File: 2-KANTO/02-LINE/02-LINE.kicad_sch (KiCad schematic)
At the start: 74 parts, among them J2 WRITER CONN, J3 Conn_01x05, U1 STM32F446RETx

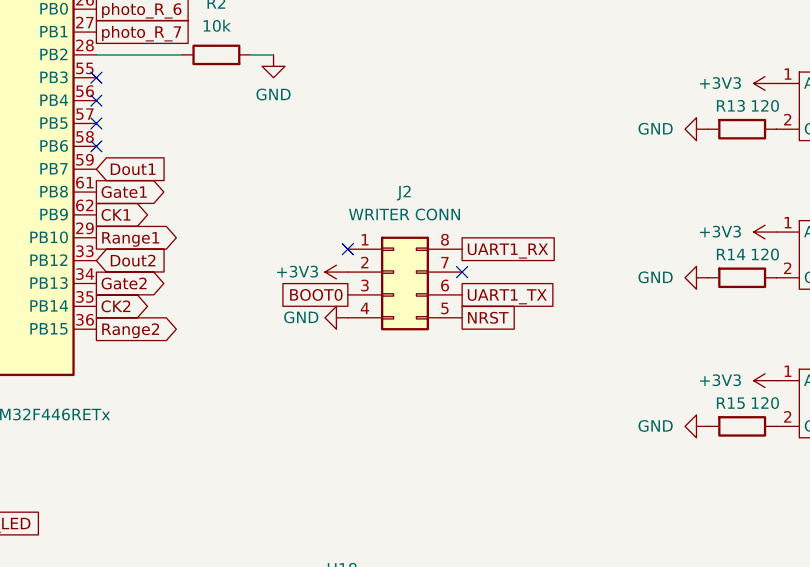
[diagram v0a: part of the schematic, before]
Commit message: mike
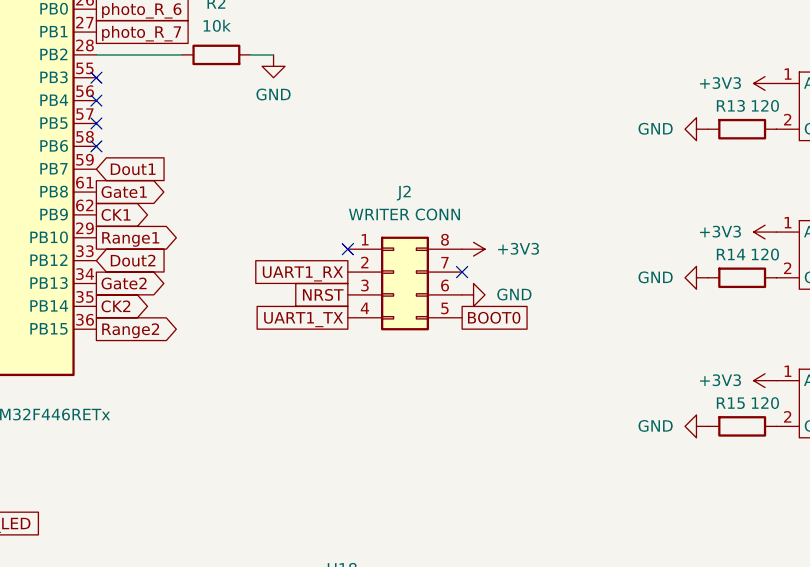
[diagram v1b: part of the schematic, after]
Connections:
- net +3V3: now also J2.8 (Pin_8); no longer J2.2 (Pin_2)
- net BOOT0: now also J2.5 (Pin_5); no longer J2.3 (Pin_3)
- net GND: now also J2.6 (Pin_6); no longer J2.4 (Pin_4)
- net NRST: now also J2.3 (Pin_3); no longer J2.5 (Pin_5)
- net UART1_RX: now also J2.2 (Pin_2); no longer J2.8 (Pin_8)
- net UART1_TX: now also J2.4 (Pin_4); no longer J2.6 (Pin_6)
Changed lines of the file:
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@@
     )
   )
-  (global_label "BOOT0" (shape passive) (at 113.665 124.46 180) (fields_autoplaced)
+  (global_label "UART1_TX" (shape passive) (at 113.665 127 180) (fields_autoplaced)
     (effects (font (size 1.27 1.27)) (justify right))
-    (property "Intersheetrefs" "${INTERSHEET_REFS}" (at 105.683 124.46 0)
+    (property "Intersheetrefs" "${INTERSHEET_REFS}" (at 102.7802 127 0)
       (effects (font (size 1.27 1.27)) (justify right) hide)
     )
@@
     )
   )
-  (global_label "UART1_TX" (shape passive) (at 126.365 124.46 0) (fields_autoplaced)
-    (effects (font (size 1.27 1.27)) (justify left))
-    (property "Intersheetrefs" "${INTERSHEET_REFS}" (at 137.2498 124.46 0)
-      (effects (font (size 1.27 1.27)) (justify left) hide)
-    )
-  )
   (global_label "Dout2" (shape input) (at 85.725 120.65 0) (fields_autoplaced)
     (effects (font (size 1.27 1.27)) (justify left))
@@
     )
   )
+  (global_label "BOOT0" (shape passive) (at 126.365 127 0) (fields_autoplaced)
+    (effects (font (size 1.27 1.27)) (justify left))
+    (property "Intersheetrefs" "${INTERSHEET_REFS}" (at 134.347 127 0)
+      (effects (font (size 1.27 1.27)) (justify left) hide)
+    )
+  )
   (global_label "photo_center" (shape passive) (at 85.725 59.69 0) (fields_autoplaced)
     (effects (font (size 1.27 1.27)) (justify left))
@@
     )
   )
+  (global_label "UART1_RX" (shape passive) (at 113.665 121.92 180) (fields_autoplaced)
+    (effects (font (size 1.27 1.27)) (justify right))
+    (property "Intersheetrefs" "${INTERSHEET_REFS}" (at 102.4778 121.92 0)
+      (effects (font (size 1.27 1.27)) (justify right) hide)
+    )
+  )
   (global_label "photo_front" (shape passive) (at 248.285 144.78 180) (fields_autoplaced)
     (effects (font (size 1.27 1.27)) (justify right))
@@
     )
   )
-  (global_label "NRST" (shape passive) (at 126.365 127 0) (fields_autoplaced)
-    (effects (font (size 1.27 1.27)) (justify left))
-    (property "Intersheetrefs" "${INTERSHEET_REFS}" (at 133.0165 127 0)
-      (effects (font (size 1.27 1.27)) (justify left) hide)
-    )
-  )
   (global_label "UART3_TX" (shape input) (at 152.4 175.26 180) (fields_autoplaced)
     (effects (font (size 1.27 1.27)) (justify right))
@@
     )
   )
-  (global_label "photo_R_2" (shape passive) (at 248.285 43.815 180) (fields_autoplaced)
+  (global_label "NRST" (shape passive) (at 113.665 124.46 180) (fields_autoplaced)
     (effects (font (size 1.27 1.27)) (justify right))
-    (property "Intersheetrefs" "${INTERSHEET_REFS}" (at 236.6747 43.815 0)
+    (property "Intersheetrefs" "${INTERSHEET_REFS}" (at 107.0135 124.46 0)
       (effects (font (size 1.27 1.27)) (justify right) hide)
     )
   )
-  (global_label "UART1_RX" (shape passive) (at 126.365 119.38 0) (fields_autoplaced)
-    (effects (font (size 1.27 1.27)) (justify left))
-    (property "Intersheetrefs" "${INTERSHEET_REFS}" (at 137.5522 119.38 0)
-      (effects (font (size 1.27 1.27)) (justify left) hide)
+  (global_label "photo_R_2" (shape passive) (at 248.285 43.815 180) (fields_autoplaced)
+    (effects (font (size 1.27 1.27)) (justify right))
+    (property "Intersheetrefs" "${INTERSHEET_REFS}" (at 236.6747 43.815 0)
+      (effects (font (size 1.27 1.27)) (justify right) hide)
     )
   )
@@
     )
   )
+  (symbol (lib_id "power:GND") (at 126.365 124.46 90) (unit 1)
+    (in_bom yes) (on_board yes) (dnp no) (fields_autoplaced)
+    (property "Reference" "#PWR013" (at 132.715 124.46 0)
+      (effects (font (size 1.27 1.27)) hide)
+    )
+    (property "Value" "GND" (at 130.175 124.46 90)
+      (effects (font (size 1.27 1.27)) (justify right))
+    )
+    (property "Footprint" "" (at 126.365 124.46 0)
+      (effects (font (size 1.27 1.27)) hide)
+    )
+    (property "Datasheet" "" (at 126.365 124.46 0)
+      (effects (font (size 1.27 1.27)) hide)
+    )
+    (pin "1")
+    (instances
+      (project "04-line_sub"
+        (path "/25c57c6f-8e34-4d58-aed4-7bf8583eb86f"
+          (reference "#PWR013") (unit 1)
+        )
+      )
+      (project "02-LINE"
+        (path "/35ef3fba-f15f-441c-9d76-e36f38a0c8a3"
+          (reference "#PWR013") (unit 1)
+        )
+      )
+      (project "06_WRITER"
+        (path "/816205b3-19fd-426f-b76d-aedd327993fe"
+          (reference "#PWR03") (unit 1)
+        )
+      )
+      (project "04-line"
+        (path "/b1a90ee4-5853-45f0-85ec-cbfa3ae36592"
+          (reference "#PWR078") (unit 1)
+        )
+      )
+    )
+  )
   (symbol (lib_id "Device:R") (at 221.615 40.005 270) (unit 1)
     (in_bom yes) (on_board yes) (dnp no)
@@
     )
   )
+  (symbol (lib_id "power:+3V3") (at 126.365 119.38 270) (unit 1)
+    (in_bom yes) (on_board yes) (dnp no) (fields_autoplaced)
+    (property "Reference" "#PWR012" (at 122.555 119.38 0)
+      (effects (font (size 1.27 1.27)) hide)
+    )
+    (property "Value" "+3V3" (at 130.175 119.38 90)
+      (effects (font (size 1.27 1.27)) (justify left))
+    )
+    (property "Footprint" "" (at 126.365 119.38 0)
+      (effects (font (size 1.27 1.27)) hide)
+    )
+    (property "Datasheet" "" (at 126.365 119.38 0)
+      (effects (font (size 1.27 1.27)) hide)
+    )
+    (pin "1")
+    (instances
+      (project "04-line_sub"
+        (path "/25c57c6f-8e34-4d58-aed4-7bf8583eb86f"
+          (reference "#PWR012") (unit 1)
+        )
+      )
+      (project "02-LINE"
+        (path "/35ef3fba-f15f-441c-9d76-e36f38a0c8a3"
+          (reference "#PWR012") (unit 1)
+        )
+      )
+      (project "06_WRITER"
+        (path "/816205b3-19fd-426f-b76d-aedd327993fe"
+          (reference "#PWR01") (unit 1)
+        )
+      )
+      (project "04-line"
+        (path "/b1a90ee4-5853-45f0-85ec-cbfa3ae36592"
+          (reference "#PWR077") (unit 1)
+        )
+      )
+    )
+  )
   (symbol (lib_id "power:+3V3") (at 102.87 161.925 90) (unit 1)
     (in_bom yes) (on_board yes) (dnp no) (fields_autoplaced)
@@
     )
   )
-  (symbol (lib_id "power:+3V3") (at 113.665 121.92 90) (unit 1)
-    (in_bom yes) (on_board yes) (dnp no) (fields_autoplaced)
-    (property "Reference" "#PWR012" (at 117.475 121.92 0)
-      (effects (font (size 1.27 1.27)) hide)
-    )
-    (property "Value" "+3V3" (at 110.49 121.92 90)
-      (effects (font (size 1.27 1.27)) (justify left))
-    )
-    (property "Footprint" "" (at 113.665 121.92 0)
-      (effects (font (size 1.27 1.27)) hide)
-    )
-    (property "Datasheet" "" (at 113.665 121.92 0)
-      (effects (font (size 1.27 1.27)) hide)
-    )
-    (pin "1")
-    (instances
-      (project "04-line_sub"
-        (path "/25c57c6f-8e34-4d58-aed4-7bf8583eb86f"
-          (reference "#PWR012") (unit 1)
-        )
-      )
-      (project "02-LINE"
-        (path "/35ef3fba-f15f-441c-9d76-e36f38a0c8a3"
-          (reference "#PWR014") (unit 1)
-        )
-      )
-      (project "06_WRITER"
-        (path "/816205b3-19fd-426f-b76d-aedd327993fe"
-          (reference "#PWR01") (unit 1)
-        )
-      )
-      (project "04-line"
-        (path "/b1a90ee4-5853-45f0-85ec-cbfa3ae36592"
-          (reference "#PWR077") (unit 1)
-        )
-      )
-    )
-  )
   (symbol (lib_id "Device:C") (at 59.055 34.925 0) (unit 1)
     (in_bom yes) (on_board yes) (dnp no)
@@
         )
       )
-    )
-  )
-  (symbol (lib_id "power:GND") (at 113.665 127 270) (unit 1)
-    (in_bom yes) (on_board yes) (dnp no) (fields_autoplaced)
-    (property "Reference" "#PWR013" (at 107.315 127 0)
-      (effects (font (size 1.27 1.27)) hide)
-    )
-    (property "Value" "GND" (at 110.49 127 90)
-      (effects (font (size 1.27 1.27)) (justify right))
-    )
-    (property "Footprint" "" (at 113.665 127 0)
-      (effects (font (size 1.27 1.27)) hide)
-    )
-    (property "Datasheet" "" (at 113.665 127 0)
-      (effects (font (size 1.27 1.27)) hide)
-    )
-    (pin "1")
-    (instances
-      (project "04-line_sub"
-        (path "/25c57c6f-8e34-4d58-aed4-7bf8583eb86f"
-          (reference "#PWR013") (unit 1)
-        )
-      )
-      (project "02-LINE"
-        (path "/35ef3fba-f15f-441c-9d76-e36f38a0c8a3"
-          (reference "#PWR015") (unit 1)
-        )
-      )
-      (project "06_WRITER"
-        (path "/816205b3-19fd-426f-b76d-aedd327993fe"
-          (reference "#PWR03") (unit 1)
-        )
-      )
-      (project "04-line"
-        (path "/b1a90ee4-5853-45f0-85ec-cbfa3ae36592"
-          (reference "#PWR078") (unit 1)
-        )
-      )
